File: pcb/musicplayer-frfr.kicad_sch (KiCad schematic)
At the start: 23 parts, among them J1 Battery, J2 AudioPlug3, J3 Display, SW1 SW_Push, SW2 SW_Push, SW3 SW_Push, SW4 RotaryEncoder_Switch, SW5 SW_SPDT, U1 XIAO-RP2350-SMD, U2 TP4056-42-ESOP8, U3 DFPLAYER_MINI

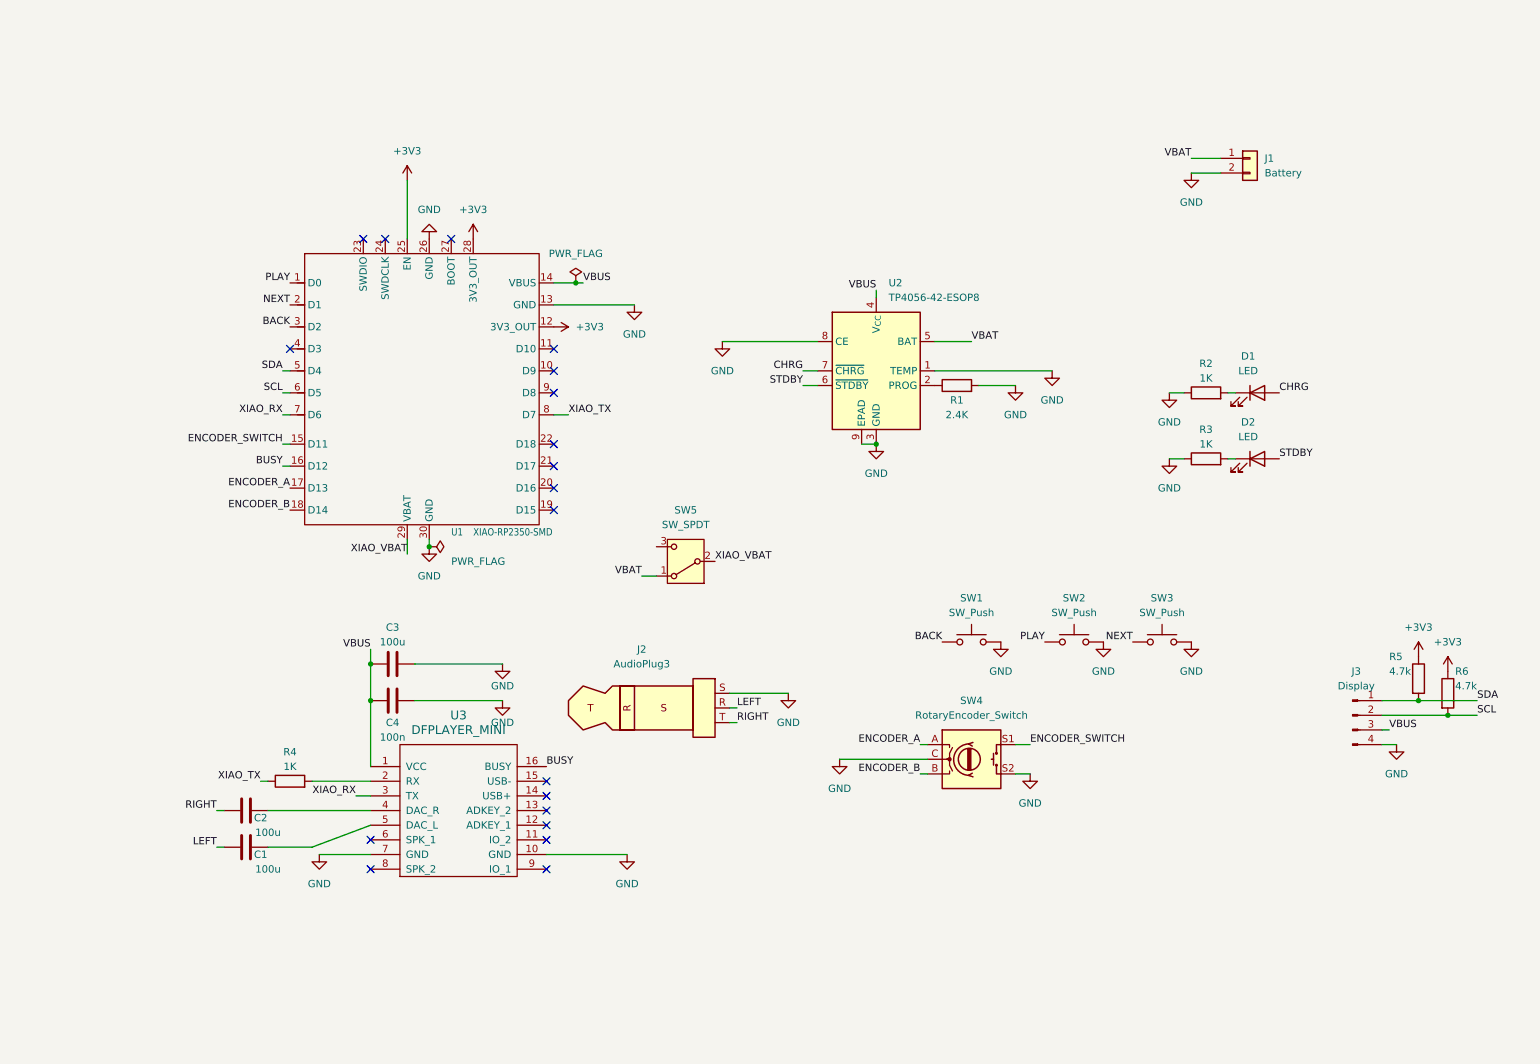
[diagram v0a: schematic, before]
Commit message: rework schemtaic to bet bigger badder and better
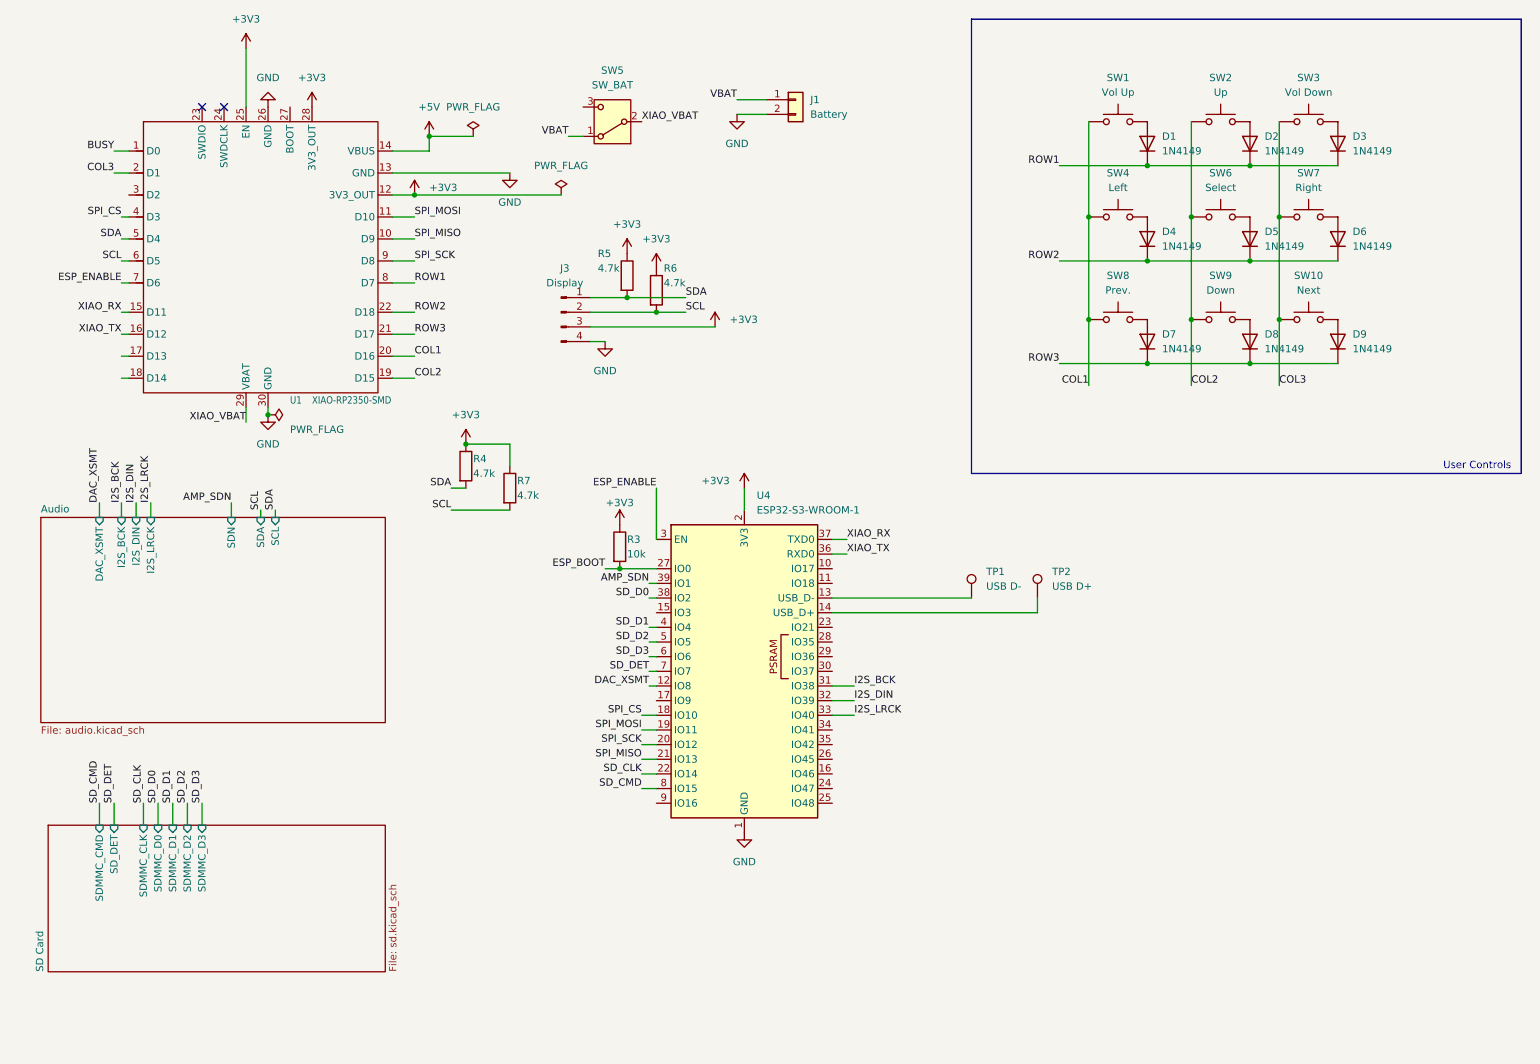
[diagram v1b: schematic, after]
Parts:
- removed C1, C2, C3: 100u, Capacitor_THT:CP_Radial_D6.3mm_P2.50mm, symbol Device:C
- removed C4: 100n, Capacitor_SMD:C_0805_2012Metric, symbol Device:C
- removed D1, D2: LED, LED_SMD:LED_0805_2012Metric, symbol Device:LED
- removed J2: AudioPlug3, Connector_Audio:Jack_3.5mm_CUI_SJ-3523-SMT_Horizontal, symbol Connector_Audio:AudioPlug3
- removed R1: 2.4K, Resistor_SMD:R_0805_2012Metric, symbol Device:R
- removed R2: 1K, Resistor_SMD:R_0805_2012Metric, symbol Device:R
- removed SW4: RotaryEncoder_Switch, Rotary_Encoder:RotaryEncoder_Alps_EC11E-Switch_Vertical_H20mm, symbol Device:RotaryEncoder_Switch
- removed U2: TP4056-42-ESOP8, Package_SO:SOIC-8-1EP_3.9x4.9mm_P1.27mm_EP2.41x3.3mm_ThermalVias, symbol Battery_Management:TP4056-42-ESOP8
- removed U3: DFPLAYER_MINI, DFPlayer:DFPlayer_V2, symbol Arduino:DFPLAYER_MINI
- added D1, D2, D3, D4, D5, D6, D7, D8, D9: 1N4149, Diode_THT:D_DO-35_SOD27_P7.62mm_Horizontal, symbol Diode:1N4149
- added R7: 4.7k, symbol Device:R
- added SW10: Next, Button_Switch_THT:SW_PUSH_6mm, symbol Switch:SW_Push
- added SW4: Left, Button_Switch_THT:SW_PUSH_6mm, symbol Switch:SW_Push
- added SW6: Select, Button_Switch_THT:SW_PUSH_6mm, symbol Switch:SW_Push
- added SW7: Right, Button_Switch_THT:SW_PUSH_6mm, symbol Switch:SW_Push
- added SW8: Prev., Button_Switch_THT:SW_PUSH_6mm, symbol Switch:SW_Push
- added SW9: Down, Button_Switch_THT:SW_PUSH_6mm, symbol Switch:SW_Push
- added TP1: USB D-, symbol Connector:TestPoint
- added TP2: USB D+, symbol Connector:TestPoint
- added U4: ESP32-S3-WROOM-1, RF_Module:ESP32-S3-WROOM-1, symbol RF_Module:ESP32-S3-WROOM-1
- R3: value 1K -> 10k; footprint Resistor_SMD:R_0805_2012Metric -> (none); LCSC PN C844939 -> (none); MPN CRCW08051K00FKEA -> (none)
- R4: value 1K -> 4.7k; footprint Resistor_SMD:R_0805_2012Metric -> (none); LCSC PN C844939 -> (none); MPN CRCW08051K00FKEA -> (none)
- SW1: value SW_Push -> Vol Up
- SW2: value SW_Push -> Up
- SW3: value SW_Push -> Vol Down
- SW5: value SW_SPDT -> SW_BAT
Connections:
- net ENCODER_SWITCH is gone; now on net XIAO_RX: U1.15 (D11)
- net +3V3: now also J3.3 (VCC), R3.1, R4.1, R7.1, U4.2 (3V3)
- net BUSY: now also U1.1 (D0); no longer U1.16 (D12)
- net GND: now also U4.1 (GND), U4.40 (GND), U4.41 (GND); no longer R3.1, SW1.2, SW2.2, SW3.2
- net SCL: now also R7.2
- net SDA: now also R4.2
- net XIAO_RX: now also U4.37 (TXD0); no longer U1.7 (D6)
- net XIAO_TX: now also U1.16 (D12), U4.36 (RXD0); no longer R4.1, U1.8 (D7)
- net SPI_MISO: now reaches U1.10 (D9)
- net SPI_MISO: now also U4.21 (IO13)
- net SPI_MOSI: now reaches U1.11 (D10)
- net SPI_MOSI: now also U4.19 (IO11)
- net COL2: now reaches U1.19 (D15)
- net COL2: now also SW2.1, SW6.1, SW9.1
- net COL1: now reaches U1.20 (D16)
- net COL1: now also SW1.1, SW4.1, SW8.1
- net ROW3: now reaches U1.21 (D17)
- net ROW3: now also D7.1 (K), D8.1 (K), D9.1 (K)
- net ROW2: now reaches U1.22 (D18)
- net ROW2: now also D4.1 (K), D5.1 (K), D6.1 (K)
- net SPI_CS: now reaches U1.4 (D3)
- net SPI_CS: now also U4.18 (IO10)
- net SPI_SCK: now reaches U1.9 (D8)
- net SPI_SCK: now also U4.20 (IO12)
- net ESP_BOOT: now reaches R3.2
- net ESP_BOOT: now also U4.27 (IO0)
- net BACK: no longer names the net of U1.3 (D2)
- net BACK: no longer SW1.1
- net ENCODER_A: no longer names the net of U1.17 (D13)
- net ENCODER_B: no longer names the net of U1.18 (D14)
- net NEXT renamed COL3
- net COL3: now also SW10.1, SW7.1
- removed net PLAY: SW2.1, U1.1 (D0)
- net VBUS renamed +5V
- net +5V: no longer J3.3 (VCC)
- new net: D1.2 (A), SW1.2
- new net: D8.2 (A), SW9.2
- new net: D9.2 (A), SW10.2
- new net: D2.2 (A), SW2.2
- new net: TP1.1, U4.13 (USB_D-)
- new net: D5.2 (A), SW6.2
- new net: D4.2 (A), SW4.2
- new net: D6.2 (A), SW7.2
- new net: D7.2 (A), SW8.2
- new net: D3.2 (A), SW3.2
- new net: TP2.1, U4.14 (USB_D+)
- new net AMP_SDN: U4.39 (IO1)
- new net DAC_XSMT: U4.12 (IO8)
- new net ESP_ENABLE: U1.7 (D6), U4.3 (EN)
- new net I2S_BCK: U4.31 (IO38)
- new net I2S_DIN: U4.32 (IO39)
- new net I2S_LRCK: U4.33 (IO40)
- new net ROW1: D1.1 (K), D2.1 (K), D3.1 (K), U1.8 (D7)
- new net SD_CLK: U4.22 (IO14)
- new net SD_CMD: U4.8 (IO15)
- new net SD_D0: U4.38 (IO2)
- new net SD_D1: U4.4 (IO4)
- new net SD_D2: U4.5 (IO5)
- new net SD_D3: U4.6 (IO6)
- new net SD_DET: U4.7 (IO7)
- no-connect marks 19 -> 2
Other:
- added sheet Audio (audio.kicad_sch)
- added sheet SD Card (sd.kicad_sch)
- note added: "User Controls"
- moved on the sheet: J1, J3, R5, R6, SW1, SW2, SW3, SW5

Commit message: add RTC and stuff
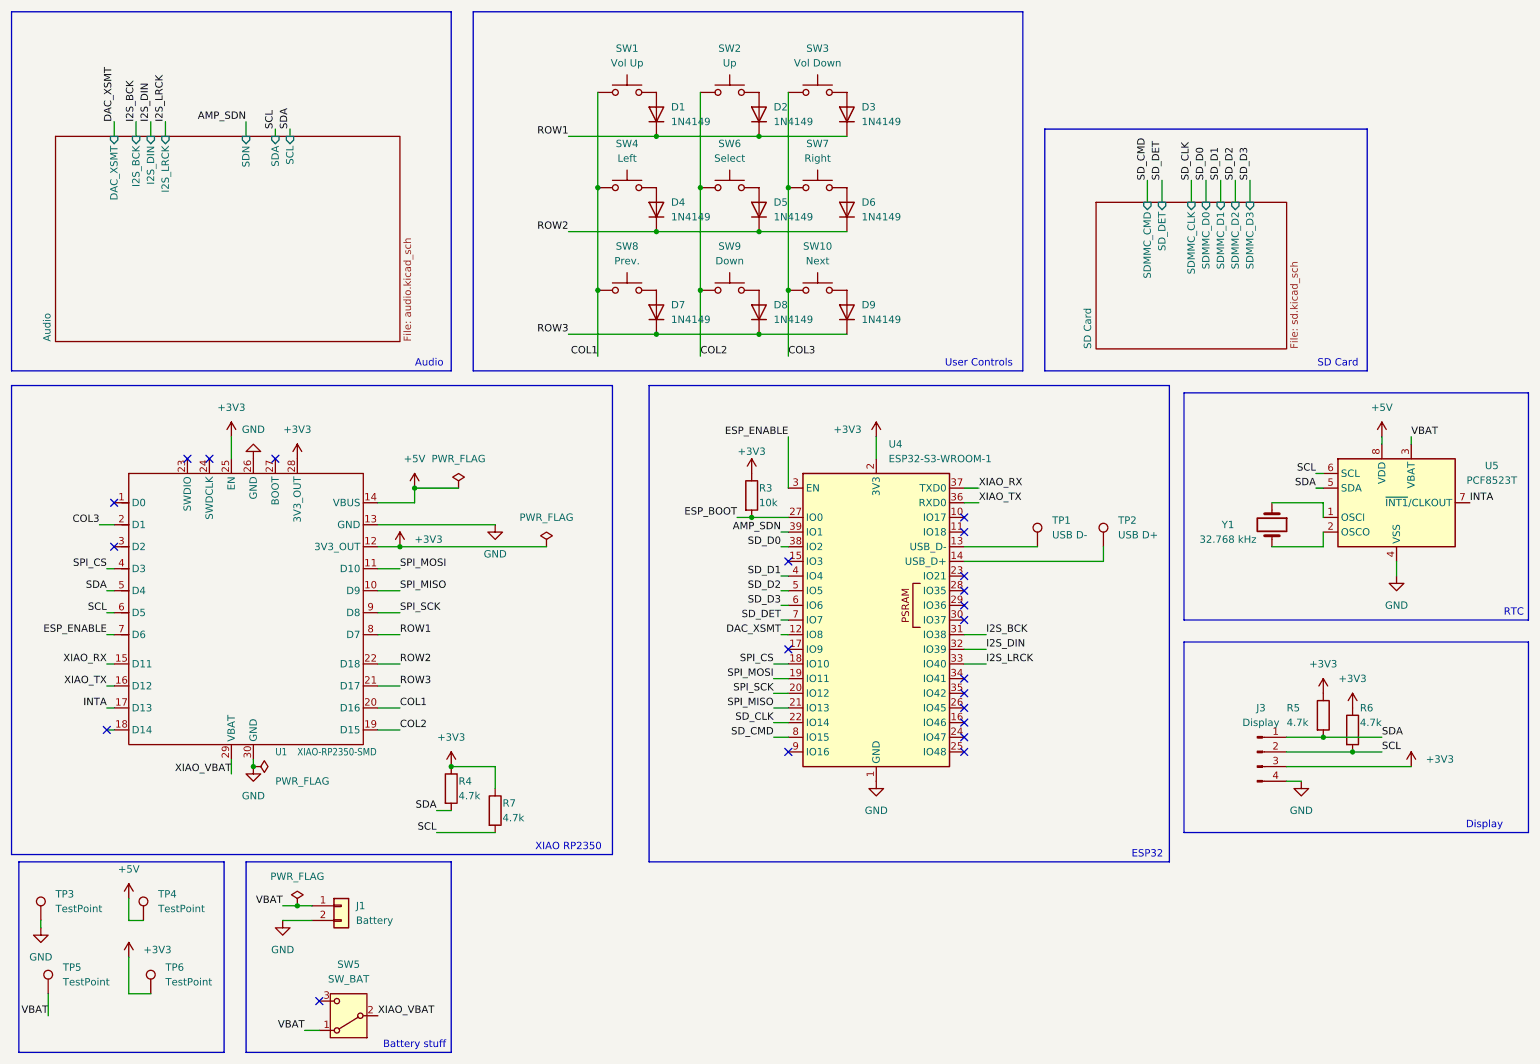
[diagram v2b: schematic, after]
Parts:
- added TP3, TP4, TP5, TP6: TestPoint, symbol Connector:TestPoint
- added U5: PCF8523T, Package_SO:SOIC-8_3.9x4.9mm_P1.27mm, symbol Timer_RTC:PCF8523T
- added Y1: 32.768 kHz, symbol Device:Crystal
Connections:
- net +3V3: now also TP6.1
- net +5V: now also TP4.1, U5.8 (VDD)
- net GND: now also TP3.1, U5.4 (VSS)
- net SCL: now also U5.6 (SCL)
- net SDA: now also U5.5 (SDA)
- net VBAT: now also TP5.1, U5.3 (VBAT)
- net INTA: now reaches U1.17 (D13)
- net INTA: now also U5.7 (~{INT1}/CLKOUT)
- net BUSY: no longer names the net of U1.1 (D0)
- new net: U5.1 (OSCI), Y1.1
- new net: U5.2 (OSCO), Y1.2
- no-connect marks 2 -> 22
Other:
- note added: "Audio"
- note added: "Battery stuff"
- note added: "Display"
- note added: "ESP32"
- note added: "RTC"
- note added: "SD Card"
- note added: "XIAO RP2350"
- moved on the sheet: D1, D2, D3, D4, D5, D6, D7, D8, D9, J1, J3, R3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
